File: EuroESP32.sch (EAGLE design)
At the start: 125 parts, among them IC1 TL074D, IC10 MCP6004, IC2 TL072, IC3 TL072, IC4 WM8731, IC5 TL074D, IC7 ADP7118, P1 A2/I34, P2 A3/I39, P3 A4/I36, P4 POWER_SIMPLE10, P5 RX/IO16, P6 TX/IO17, P7 SDA, P8 SCL, P9 IO13, U1 LM4040SOT23, U2 MCP3204-CI/SL

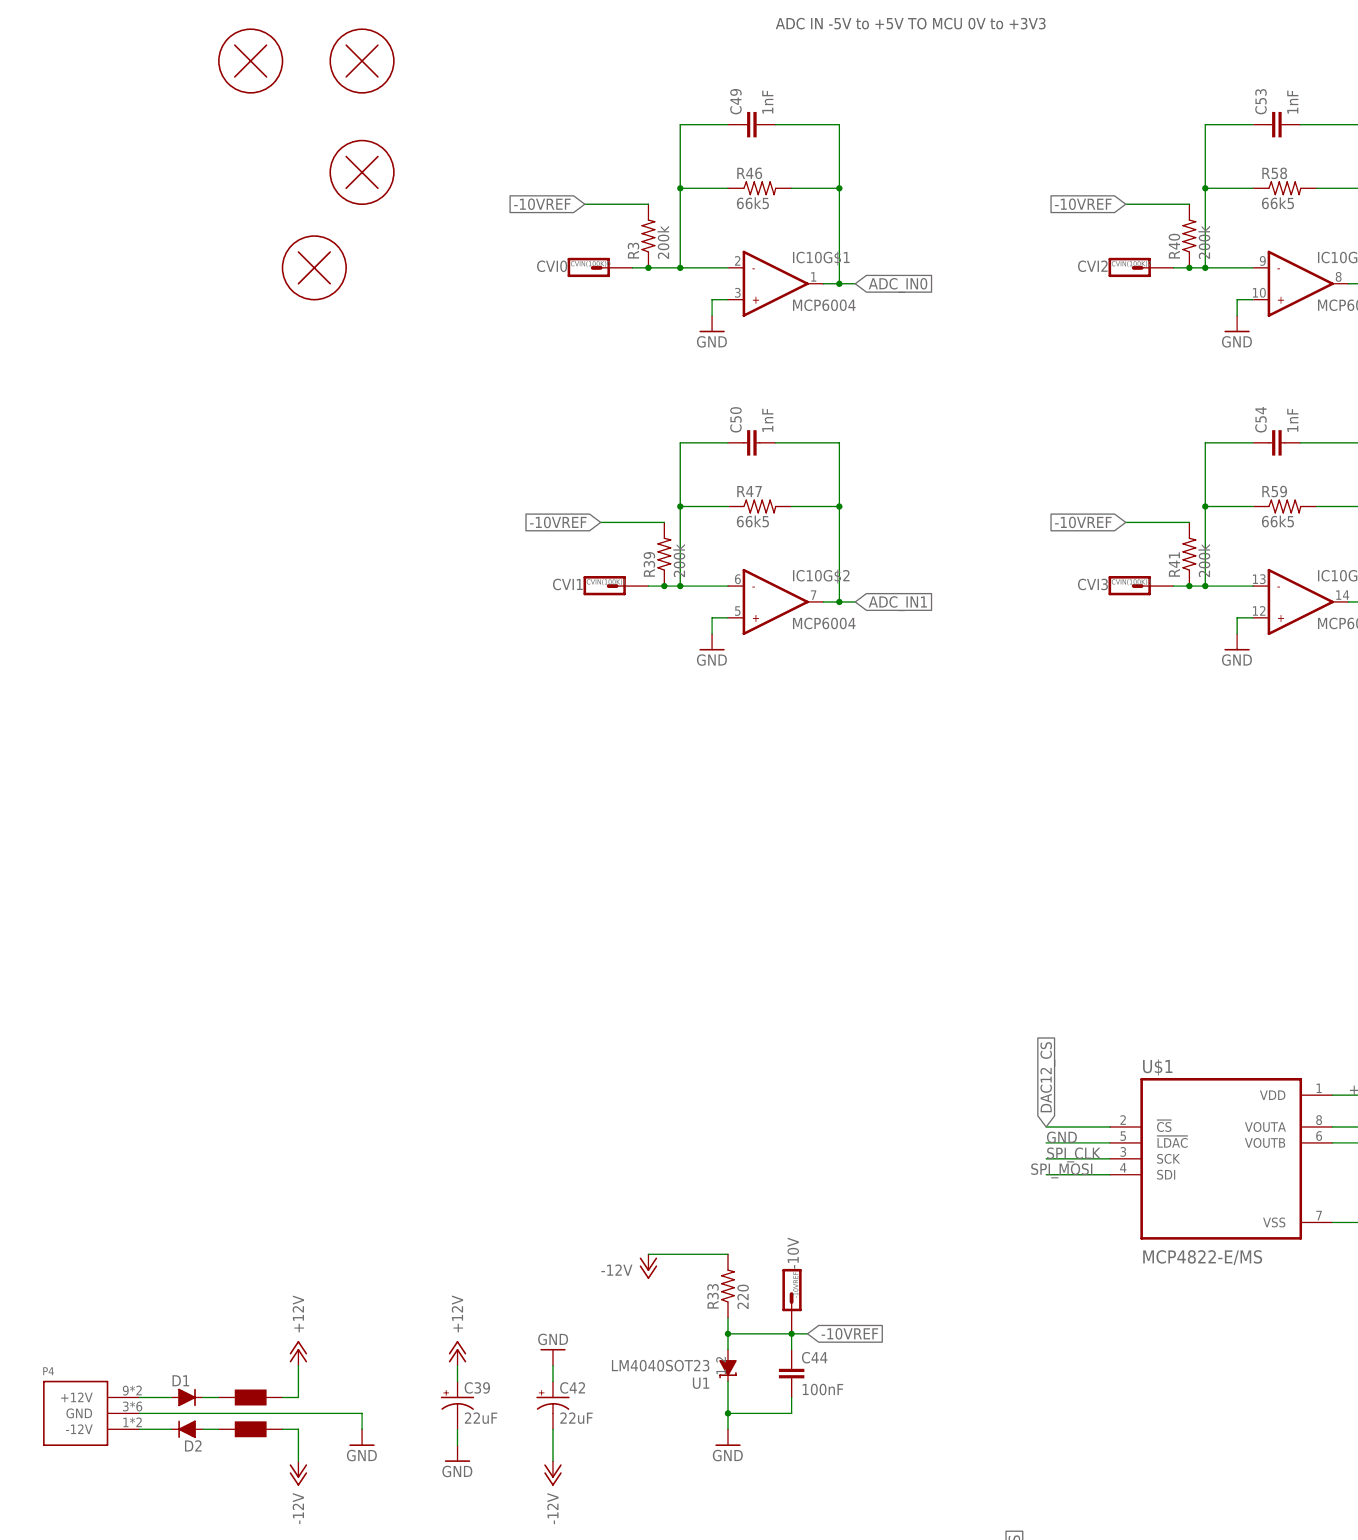
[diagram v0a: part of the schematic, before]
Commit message: Added a little information
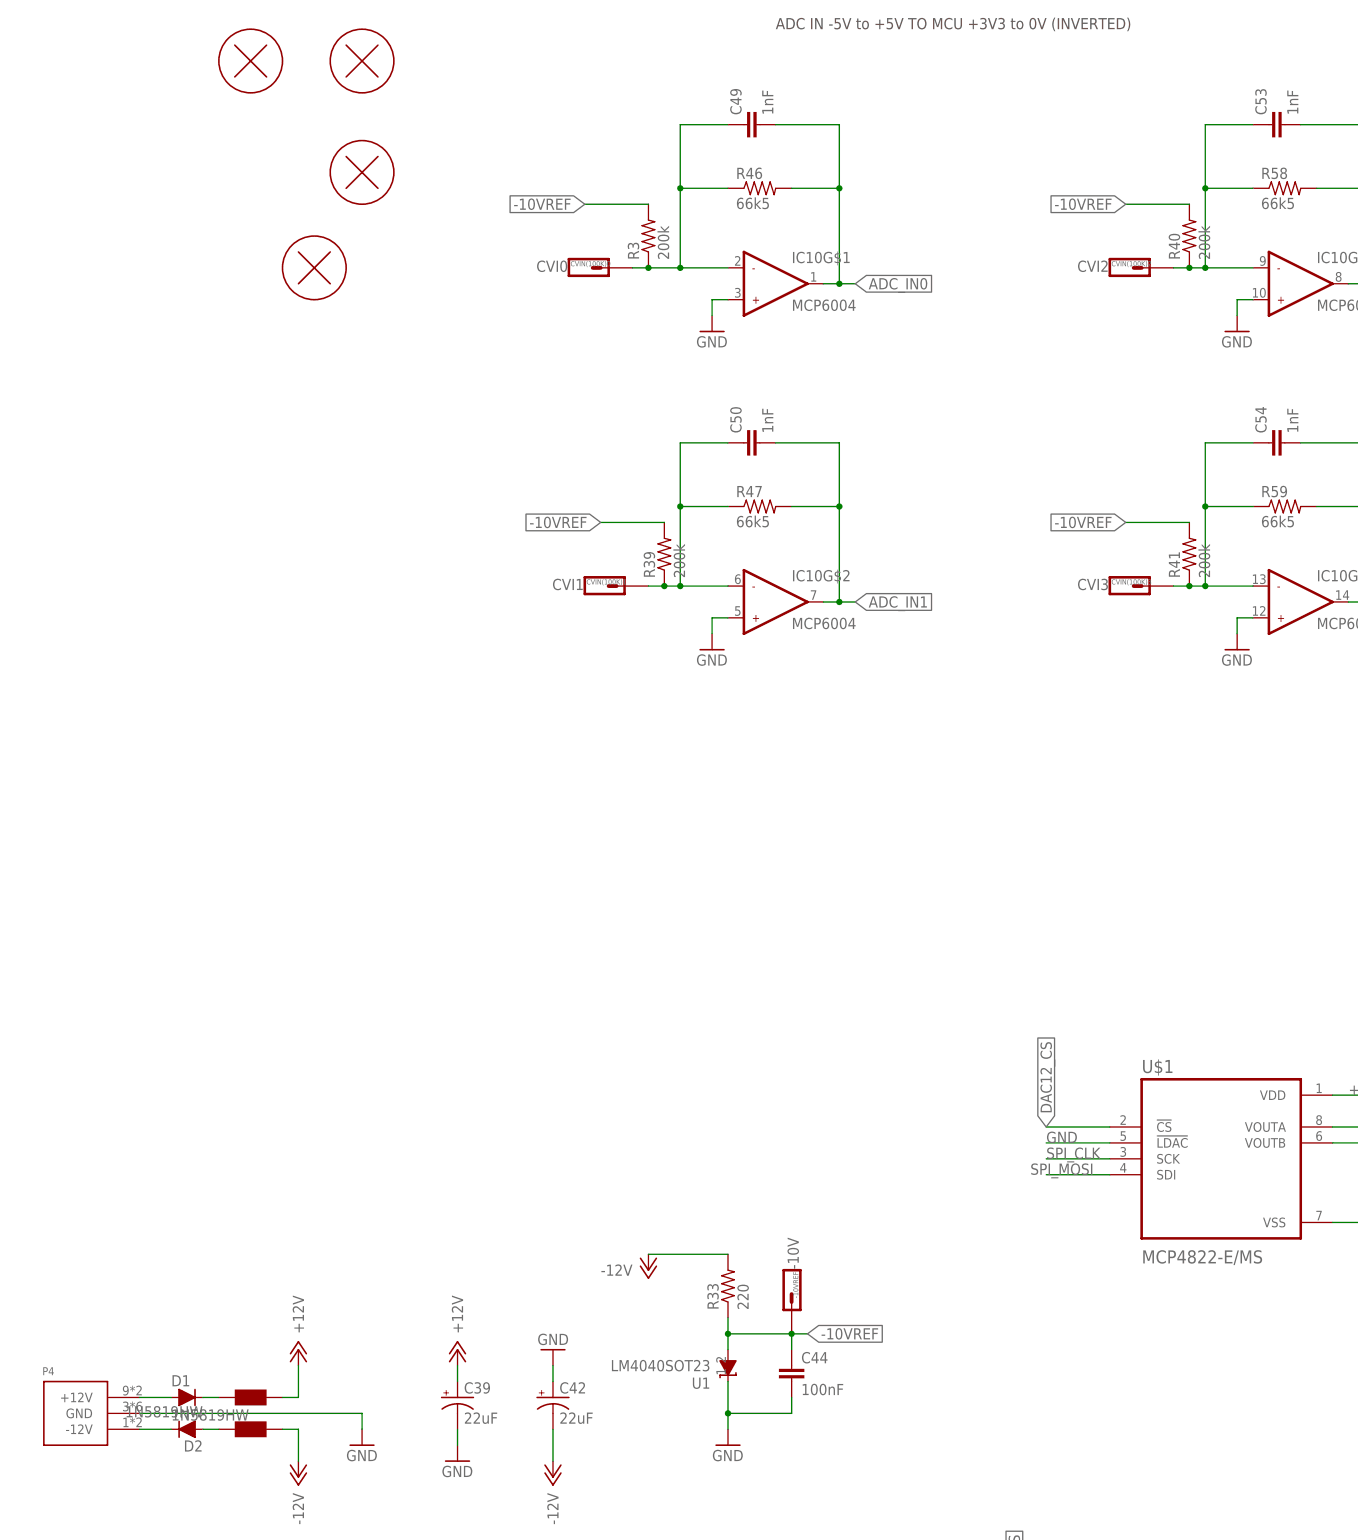
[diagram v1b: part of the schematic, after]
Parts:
- D1, D2: value (none) -> 1N5819HW
- F1, F2: value FERRITE-BEAD0805 -> Würth Electronics 742792664
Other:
- note added: "ADC IN -5V to +5V TO MCU +3V3 to 0V (INVERTED)"
- note removed: "ADC IN -5V to +5V TO MCU 0V to +3V3"
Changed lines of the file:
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@@
 <part name="GND26" library="parts_aman" deviceset="GND" device=""/>
 <part name="P4" library="parts_aman" deviceset="POWER_SIMPLE" device="10"/>
-<part name="D1" library="parts_aman" deviceset="DIODE" device=""/>
-<part name="D2" library="parts_aman" deviceset="DIODE" device=""/>
-<part name="F1" library="parts_aman" deviceset="FERRITE-BEAD" device="0805" value="FERRITE-BEAD0805"/>
-<part name="F2" library="parts_aman" deviceset="FERRITE-BEAD" device="0805" value="FERRITE-BEAD0805"/>
+<part name="D1" library="parts_aman" deviceset="DIODE" device="" value="1N5819HW"/>
+<part name="D2" library="parts_aman" deviceset="DIODE" device="" value="1N5819HW"/>
+<part name="F1" library="parts_aman" deviceset="FERRITE-BEAD" device="0805" value="Würth Electronics 742792664"/>
+<part name="F2" library="parts_aman" deviceset="FERRITE-BEAD" device="0805" value="Würth Electronics 742792664"/>
 <part name="P+4" library="parts_aman" deviceset="+12V" device=""/>
 <part name="P-2" library="parts_aman" deviceset="-12V" device=""/>
@@
 <sheet>
 <plain>
-<text x="241.3" y="86.36" size="1.778" layer="97" grouprefs="CV_IN">ADC IN -5V to +5V TO MCU 0V to +3V3</text>
+<text x="241.3" y="86.36" size="1.778" layer="97" grouprefs="CV_IN">ADC IN -5V to +5V TO MCU +3V3 to 0V (INVERTED)</text>
 </plain>
 <instances>
